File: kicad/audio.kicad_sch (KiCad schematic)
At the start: 4 parts, among them J2 AudioJack3_Ground, U10 OPA1622, U11 TPA6110A2DGN, U3 CS43131-CNZR

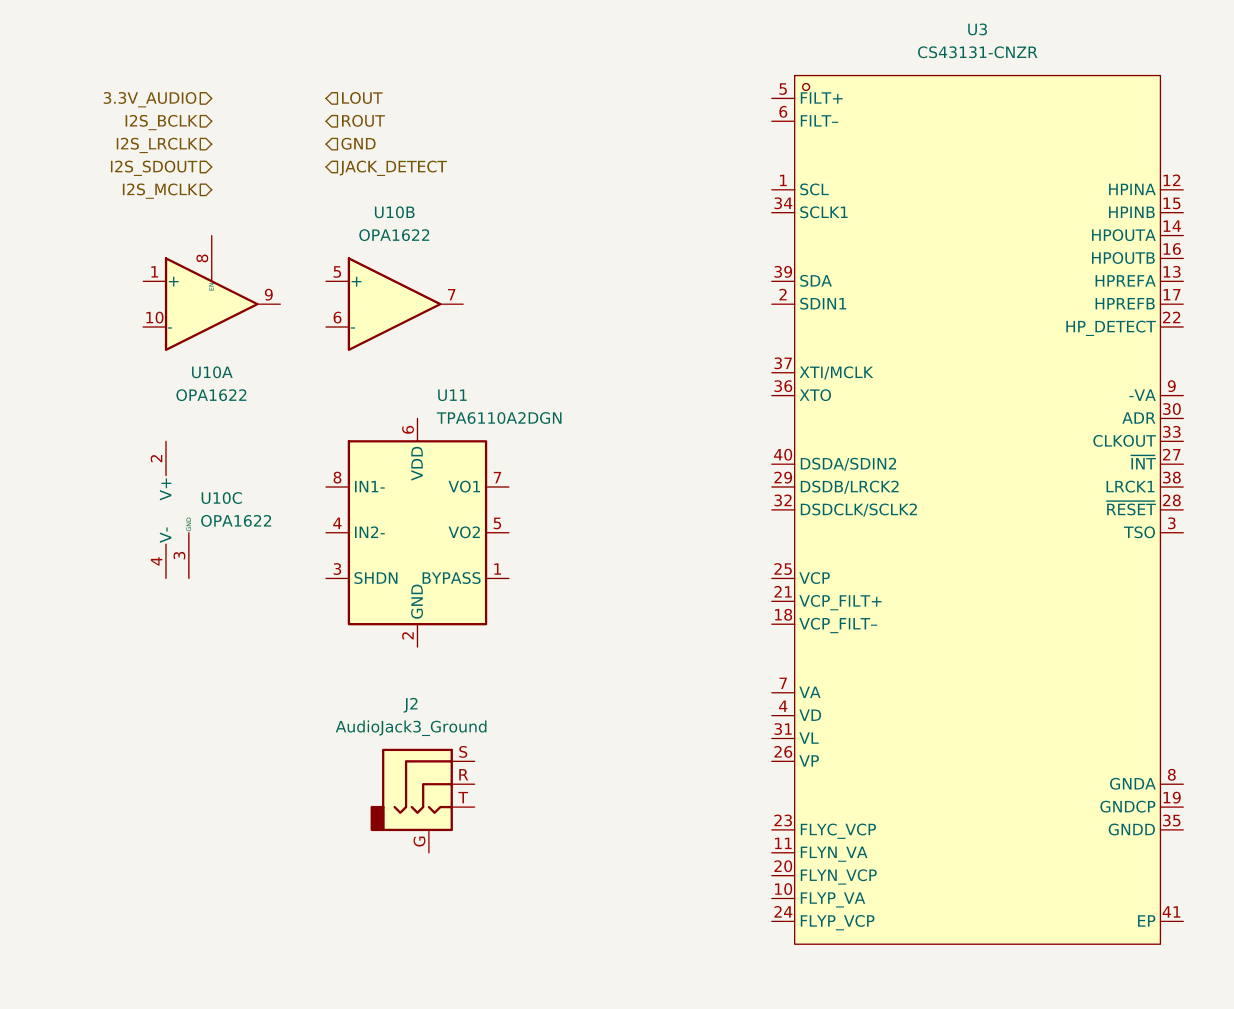
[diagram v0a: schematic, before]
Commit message: updates
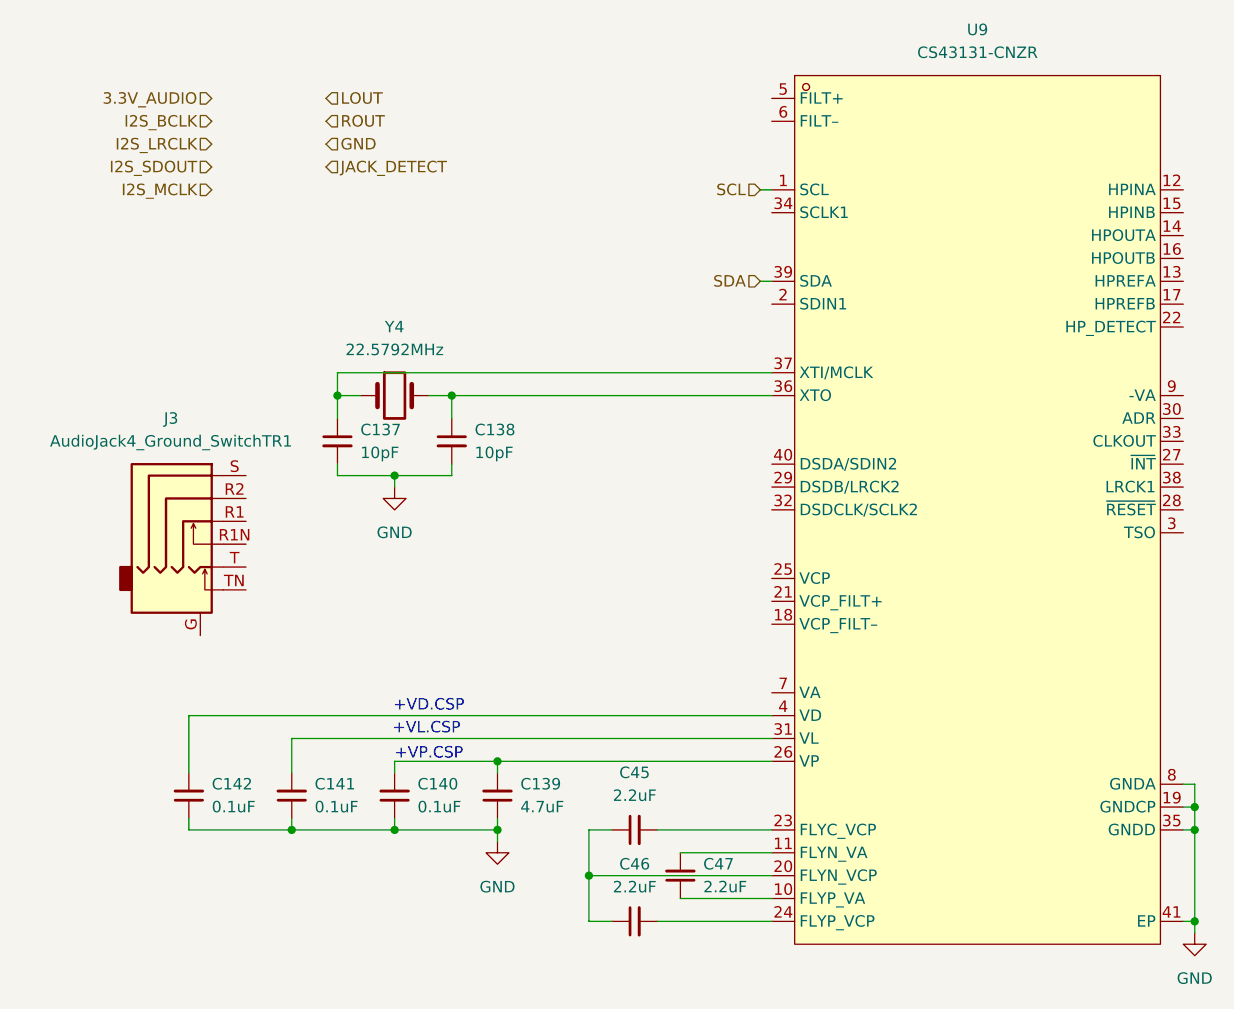
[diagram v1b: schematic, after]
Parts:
- removed J2: AudioJack3_Ground, symbol Connector_Audio:AudioJack3_Ground
- removed U10: OPA1622, Package_SON:Texas_S-PVSON-N10, symbol Amplifier_Audio:OPA1622
- removed U11: TPA6110A2DGN, Package_SO:HVSSOP-8-1EP_3x3mm_P0.65mm_EP1.57x1.89mm, symbol Amplifier_Audio:TPA6110A2DGN
- added C137, C138: 10pF, symbol Device:C_Small
- added C139: 4.7uF, symbol Device:C_Small
- added C140, C141, C142: 0.1uF, symbol Device:C_Small
- added C45, C46, C47: 2.2uF, symbol Device:C_Small
- added J3: AudioJack4_Ground_SwitchTR1, symbol Connector_Audio:AudioJack4_Ground_SwitchTR1
- added Y4: 22.5792MHz, symbol Device:Crystal
- renumbered U3 to U9
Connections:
- net GND: now also U9.19 (GNDCP), U9.35 (GNDD), U9.41 (EP), U9.8 (GNDA), C137.2, C138.2, C139.1, C140.1, C141.1, C142.1
- net SCL: now reaches U9.1 (SCL)
- net at U9.10 (FLYP_VA): now also C47.1
- net at U9.11 (FLYN_VA): now also C47.2
- net at U9.20 (FLYN_VCP): now also C45.1, C46.1
- net at U9.23 (FLYC_VCP): now also C45.2
- net at U9.24 (FLYP_VCP): now also C46.2
- net at U9.26 (VP): now also C139.2, C140.2
- net at U9.31 (VL): now also C141.2
- net at U9.36 (XTO): now also C138.1, Y4.2
- net at U9.37 (XTI/MCLK): now also C137.1, Y4.1
- net SDA: now reaches U9.39 (SDA)
- net at U9.4 (VD): now also C142.2
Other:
- note added: "+VD.CSP"
- note added: "+VL.CSP"
- note added: "+VP.CSP"
